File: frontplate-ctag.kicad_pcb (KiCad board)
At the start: 2 copper layers, 111.3 x 128.5 mm, 30 parts

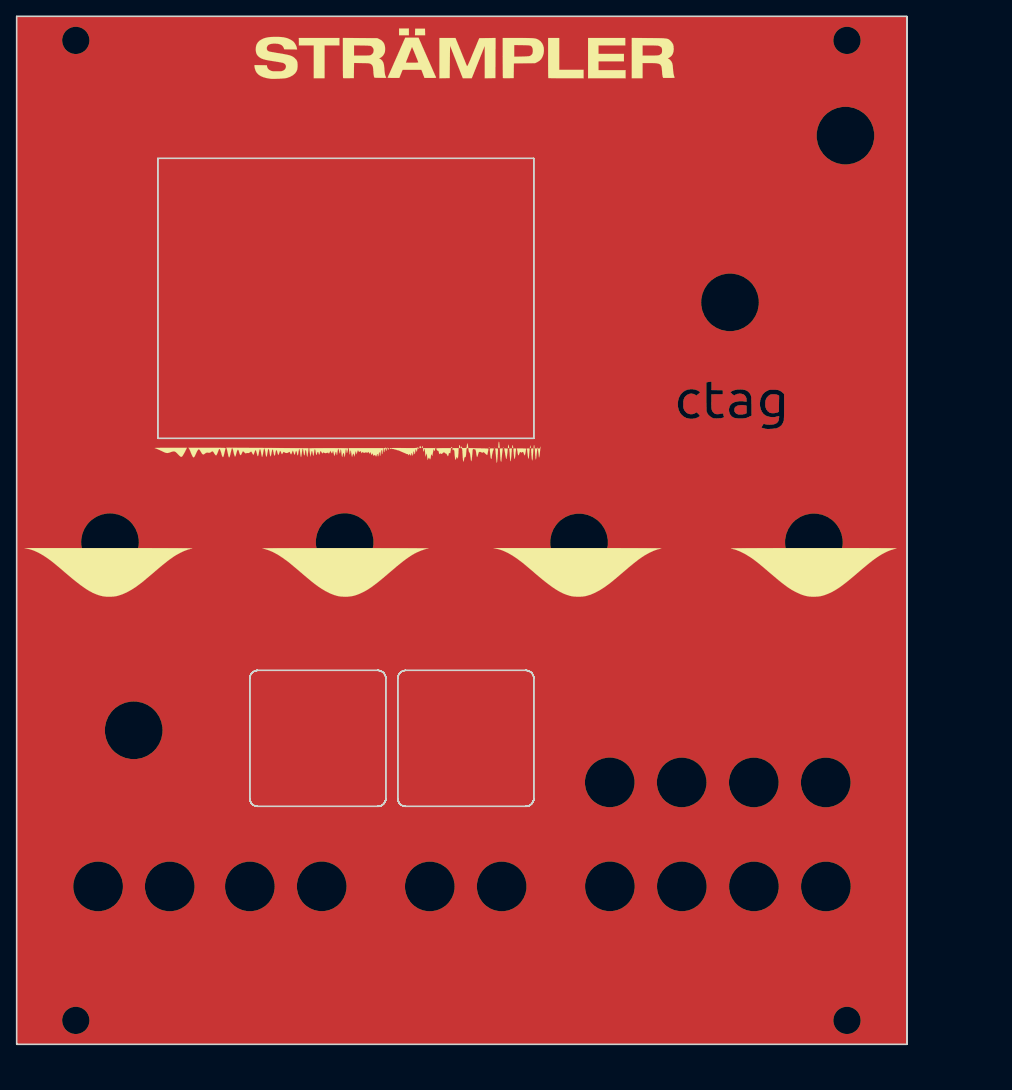
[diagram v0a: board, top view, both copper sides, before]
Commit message: cleanups and gerbers
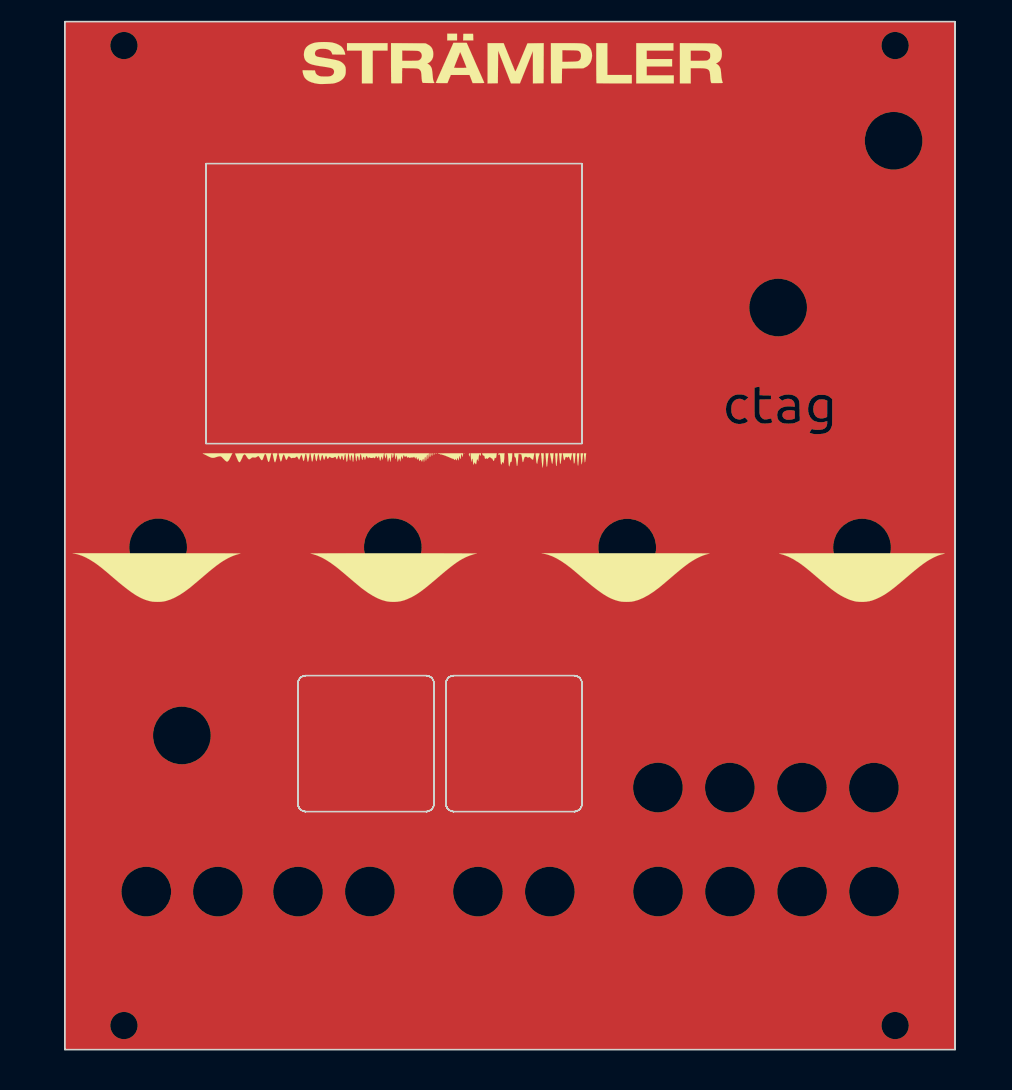
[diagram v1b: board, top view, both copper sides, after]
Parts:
- removed the ? at (145.3, 48.4)
- removed the ? at (70.8, 142.3)
- removed the ? at (79.8, 142.2)
- removed the ? at (93.3, 142.3)
- removed the ? at (102.3, 142.3)
- removed the ? at (115.8, 129.3)
- removed the ? at (124.8, 129.3)
- removed the ? at (133.8, 129.3)
- removed the ? at (142.8, 129.3)
- removed the ? at (115.8, 142.2)
- removed the ? at (124.8, 142.3)
- removed the ? at (141.3, 99.3)
- removed the ? at (133.8, 142.3)
- removed the ? at (142.8, 142.3)
- removed the ? at (145.5, 36.5)
- removed the ? at (49.1, 159.0)
- removed the ? at (145.5, 159.0)
- removed the ? at (49.1, 36.5)
- removed the ? at (112.0, 99.3)
- removed the ? at (82.7, 99.2)
- removed the ? at (53.4, 99.2)
- removed the ? at (130.9, 69.3)
- removed the ? at (56.3, 122.7)
- removed the ? at (51.9, 142.3)
- removed the ? at (60.8, 142.3)
- removed the G*** at (97.3, 97.8) (x5)
- added ?: , Wire_Pads:SolderWirePad_single_0-8mmDrill, F.Cu at (151.3, 49.1)
- added ?: , Wire_Pads:SolderWirePad_single_0-8mmDrill, F.Cu at (76.9, 142.9)
- added ?: , Wire_Pads:SolderWirePad_single_0-8mmDrill, F.Cu at (85.8, 142.9)
- added ?: , Wire_Pads:SolderWirePad_single_0-8mmDrill, F.Cu at (99.3, 142.9)
- added ?: , Wire_Pads:SolderWirePad_single_0-8mmDrill, F.Cu at (108.3, 142.9)
- added ?: , Wire_Pads:SolderWirePad_single_0-8mmDrill, F.Cu at (121.8, 129.9)
- added ?: , Wire_Pads:SolderWirePad_single_0-8mmDrill, F.Cu at (130.8, 129.9)
- added ?: , Wire_Pads:SolderWirePad_single_0-8mmDrill, F.Cu at (139.8, 129.9)
- added ?: , Wire_Pads:SolderWirePad_single_0-8mmDrill, F.Cu at (148.8, 129.9)
- added ?: , Wire_Pads:SolderWirePad_single_0-8mmDrill, F.Cu at (121.9, 142.9)
- added ?: , Wire_Pads:SolderWirePad_single_0-8mmDrill, F.Cu at (130.9, 142.9)
- added ?: , Wire_Pads:SolderWirePad_single_0-8mmDrill, F.Cu at (147.4, 99.9)
- added ?: , Wire_Pads:SolderWirePad_single_0-8mmDrill, F.Cu at (139.9, 142.9)
- added ?: , Wire_Pads:SolderWirePad_single_0-8mmDrill, F.Cu at (148.9, 142.9)
- added ?: , Wire_Pads:SolderWirePad_single_0-8mmDrill, F.Cu at (151.5, 37.1)
- added ?: , Wire_Pads:SolderWirePad_single_0-8mmDrill, F.Cu at (55.1, 159.6)
- added ?: , Wire_Pads:SolderWirePad_single_0-8mmDrill, F.Cu at (151.5, 159.6)
- added ?: , Wire_Pads:SolderWirePad_single_0-8mmDrill, F.Cu at (55.1, 37.1)
- added ?: , Wire_Pads:SolderWirePad_single_0-8mmDrill, F.Cu at (118.0, 99.9)
- added ?: , Wire_Pads:SolderWirePad_single_0-8mmDrill, F.Cu at (88.7, 99.9)
- added ?: , Wire_Pads:SolderWirePad_single_0-8mmDrill, F.Cu at (59.4, 99.9)
- added ?: , Wire_Pads:SolderWirePad_single_0-8mmDrill, F.Cu at (136.9, 69.9)
- added ?: , Wire_Pads:SolderWirePad_single_0-8mmDrill, F.Cu at (62.3, 123.4)
- added ?: , Wire_Pads:SolderWirePad_single_0-8mmDrill, F.Cu at (57.9, 142.9)
- added ?: , Wire_Pads:SolderWirePad_single_0-8mmDrill, F.Cu at (66.8, 142.9)
- added G*** (x5): LOGO, LOGO, F.Cu at (103.3, 98.4)

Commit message: sending for production
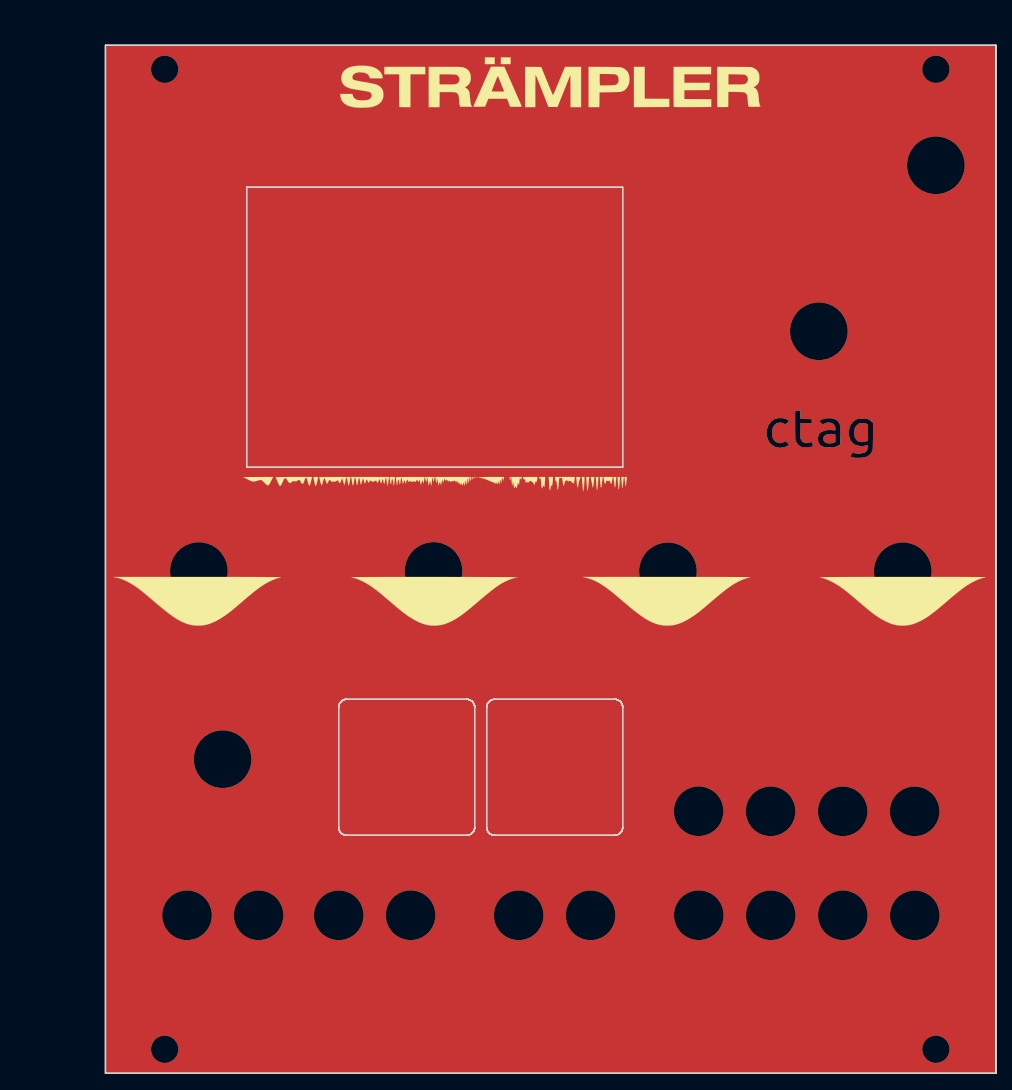
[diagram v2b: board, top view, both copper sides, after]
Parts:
- removed the ? at (151.3, 49.1)
- removed the ? at (76.9, 142.9)
- removed the ? at (85.8, 142.9)
- removed the ? at (99.3, 142.9)
- removed the ? at (108.3, 142.9)
- removed the ? at (121.8, 129.9)
- removed the ? at (130.8, 129.9)
- removed the ? at (139.8, 129.9)
- removed the ? at (148.8, 129.9)
- removed the ? at (121.9, 142.9)
- removed the ? at (130.9, 142.9)
- removed the ? at (147.4, 99.9)
- removed the ? at (139.9, 142.9)
- removed the ? at (148.9, 142.9)
- removed the ? at (151.5, 37.1)
- removed the ? at (55.1, 159.6)
- removed the ? at (151.5, 159.6)
- removed the ? at (55.1, 37.1)
- removed the ? at (118.0, 99.9)
- removed the ? at (88.7, 99.9)
- removed the ? at (59.4, 99.9)
- removed the ? at (136.9, 69.9)
- removed the ? at (62.3, 123.4)
- removed the ? at (57.9, 142.9)
- removed the ? at (66.8, 142.9)
- removed the G*** at (103.3, 98.4) (x5)
- added ?: , Wire_Pads:SolderWirePad_single_0-8mmDrill, F.Cu at (156.6, 52.1)
- added ?: , Wire_Pads:SolderWirePad_single_0-8mmDrill, F.Cu at (81.9, 145.9)
- added ?: , Wire_Pads:SolderWirePad_single_0-8mmDrill, F.Cu at (90.9, 145.9)
- added ?: , Wire_Pads:SolderWirePad_single_0-8mmDrill, F.Cu at (104.4, 145.9)
- added ?: , Wire_Pads:SolderWirePad_single_0-8mmDrill, F.Cu at (113.4, 145.9)
- added ?: , Wire_Pads:SolderWirePad_single_0-8mmDrill, F.Cu at (126.9, 132.9)
- added ?: , Wire_Pads:SolderWirePad_single_0-8mmDrill, F.Cu at (135.9, 132.9)
- added ?: , Wire_Pads:SolderWirePad_single_0-8mmDrill, F.Cu at (144.9, 132.9)
- added ?: , Wire_Pads:SolderWirePad_single_0-8mmDrill, F.Cu at (153.9, 132.9)
- added ?: , Wire_Pads:SolderWirePad_single_0-8mmDrill, F.Cu at (126.9, 145.9)
- added ?: , Wire_Pads:SolderWirePad_single_0-8mmDrill, F.Cu at (135.9, 145.9)
- added ?: , Wire_Pads:SolderWirePad_single_0-8mmDrill, F.Cu at (152.4, 102.9)
- added ?: , Wire_Pads:SolderWirePad_single_0-8mmDrill, F.Cu at (145.0, 145.9)
- added ?: , Wire_Pads:SolderWirePad_single_0-8mmDrill, F.Cu at (153.9, 145.9)
- added ?: , Wire_Pads:SolderWirePad_single_0-8mmDrill, F.Cu at (156.6, 40.1)
- added ?: , Wire_Pads:SolderWirePad_single_0-8mmDrill, F.Cu at (60.2, 162.6)
- added ?: , Wire_Pads:SolderWirePad_single_0-8mmDrill, F.Cu at (156.6, 162.6)
- added ?: , Wire_Pads:SolderWirePad_single_0-8mmDrill, F.Cu at (60.2, 40.1)
- added ?: , Wire_Pads:SolderWirePad_single_0-8mmDrill, F.Cu at (123.1, 102.9)
- added ?: , Wire_Pads:SolderWirePad_single_0-8mmDrill, F.Cu at (93.8, 102.8)
- added ?: , Wire_Pads:SolderWirePad_single_0-8mmDrill, F.Cu at (64.5, 102.8)
- added ?: , Wire_Pads:SolderWirePad_single_0-8mmDrill, F.Cu at (142.0, 72.9)
- added ?: , Wire_Pads:SolderWirePad_single_0-8mmDrill, F.Cu at (67.4, 126.4)
- added ?: , Wire_Pads:SolderWirePad_single_0-8mmDrill, F.Cu at (63.0, 145.9)
- added ?: , Wire_Pads:SolderWirePad_single_0-8mmDrill, F.Cu at (71.9, 145.9)
- added G*** (x5): LOGO, LOGO, F.Cu at (108.4, 101.4)
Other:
- board text added: "JLCJLCJLCJLC"
